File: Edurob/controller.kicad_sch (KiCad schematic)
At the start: 9 parts, among them SW1 SW_Push, U4 ESP32-S3-WROOM-1

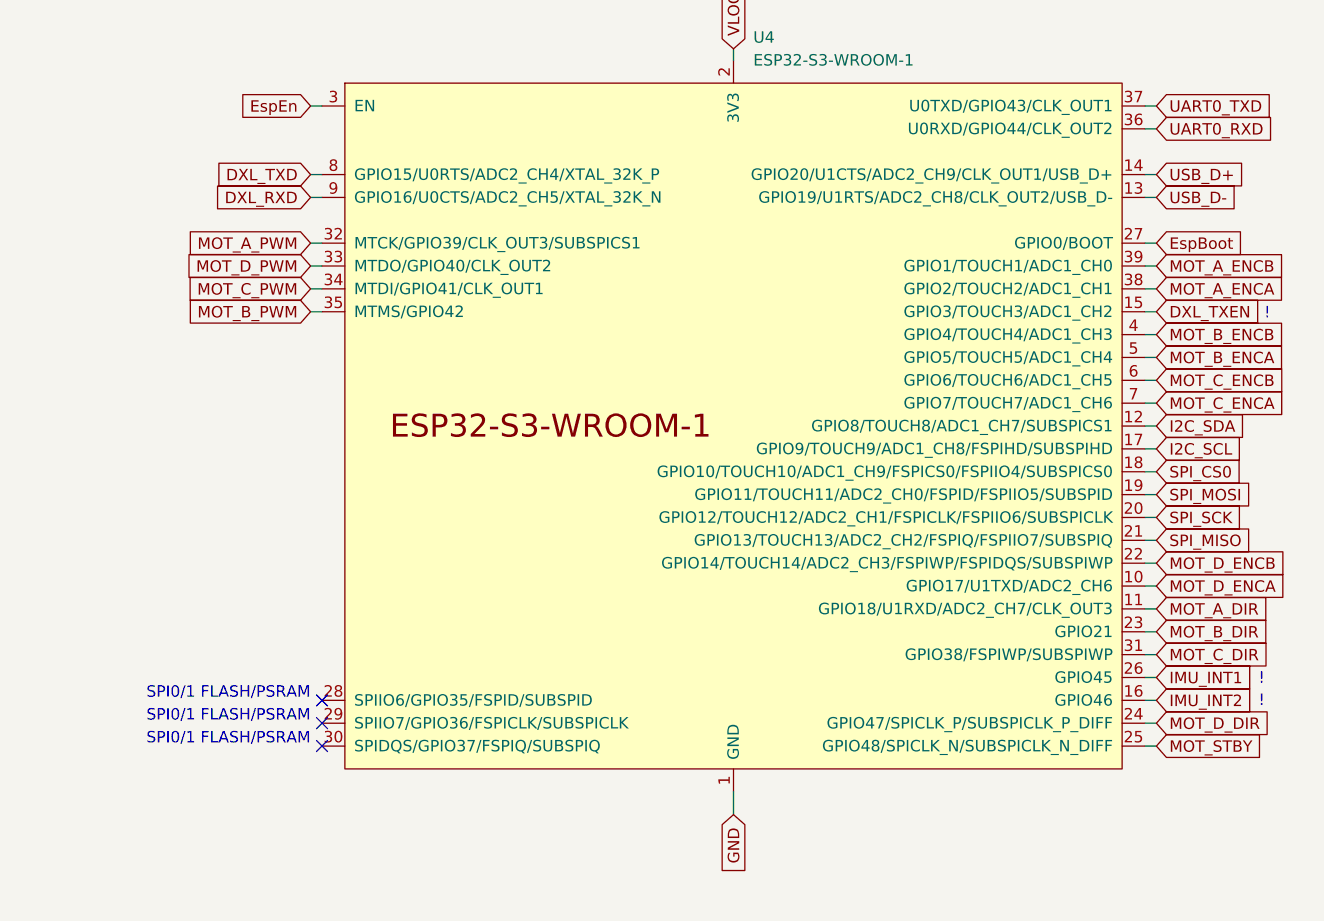
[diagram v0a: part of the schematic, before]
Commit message: Finalized part placement
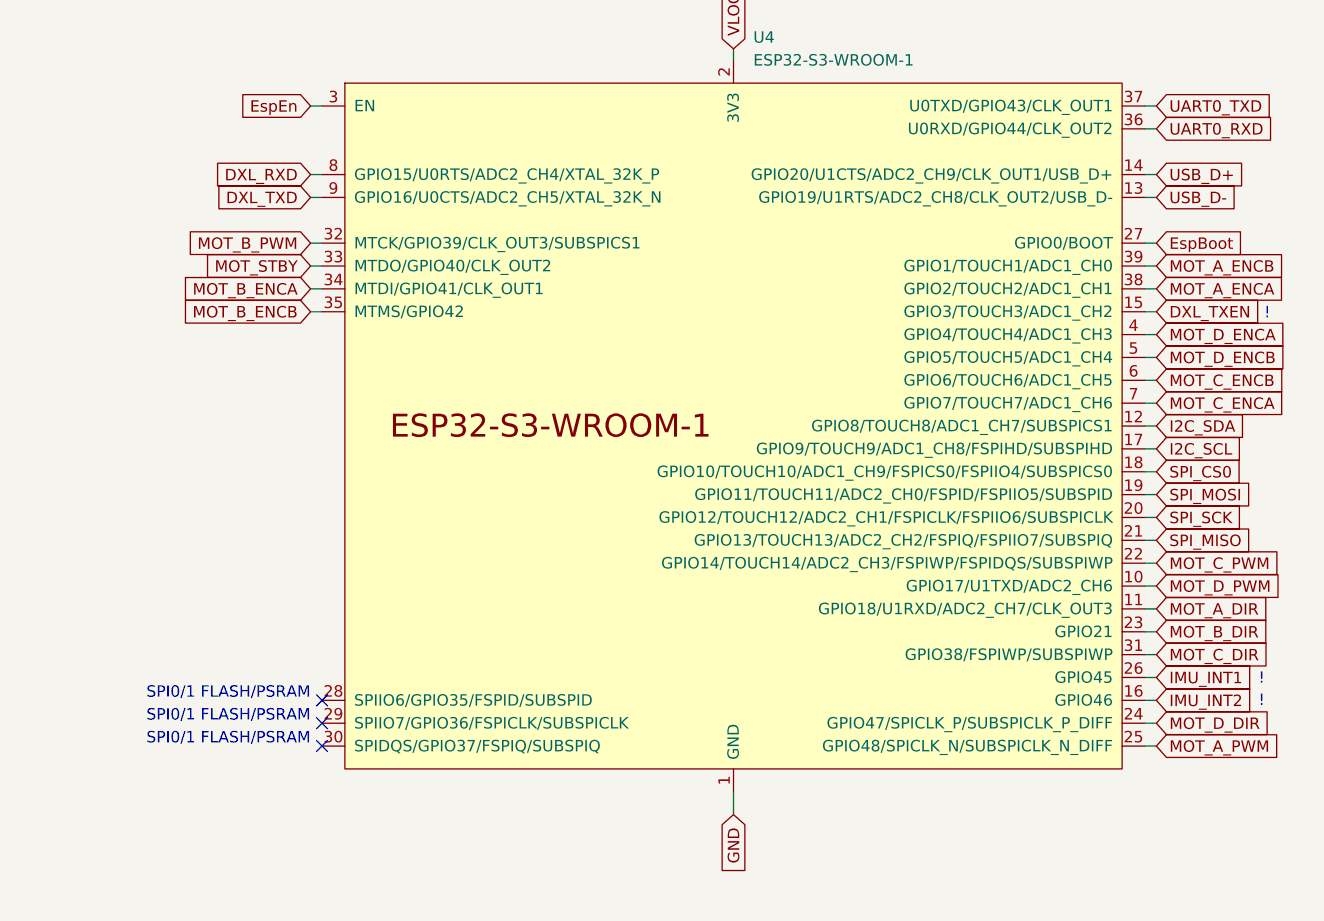
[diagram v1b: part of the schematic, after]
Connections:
- net DXL_RXD: now also U4.8 (GPIO15/U0RTS/ADC2_CH4/XTAL_32K_P); no longer U4.9 (GPIO16/U0CTS/ADC2_CH5/XTAL_32K_N)
- net DXL_TXD: now also U4.9 (GPIO16/U0CTS/ADC2_CH5/XTAL_32K_N); no longer U4.8 (GPIO15/U0RTS/ADC2_CH4/XTAL_32K_P)
- net MOT_A_PWM: now also U4.25 (GPIO48/SPICLK_N/SUBSPICLK_N_DIFF); no longer U4.32 (MTCK/GPIO39/CLK_OUT3/SUBSPICS1)
- net MOT_B_ENCA: now also U4.34 (MTDI/GPIO41/CLK_OUT1); no longer U4.5 (GPIO5/TOUCH5/ADC1_CH4)
- net MOT_B_ENCB: now also U4.35 (MTMS/GPIO42); no longer U4.4 (GPIO4/TOUCH4/ADC1_CH3)
- net MOT_B_PWM: now also U4.32 (MTCK/GPIO39/CLK_OUT3/SUBSPICS1); no longer U4.35 (MTMS/GPIO42)
- net MOT_C_PWM: now also U4.22 (GPIO14/TOUCH14/ADC2_CH3/FSPIWP/FSPIDQS/SUBSPIWP); no longer U4.34 (MTDI/GPIO41/CLK_OUT1)
- net MOT_D_ENCA: now also U4.4 (GPIO4/TOUCH4/ADC1_CH3); no longer U4.10 (GPIO17/U1TXD/ADC2_CH6)
- net MOT_D_ENCB: now also U4.5 (GPIO5/TOUCH5/ADC1_CH4); no longer U4.22 (GPIO14/TOUCH14/ADC2_CH3/FSPIWP/FSPIDQS/SUBSPIWP)
- net MOT_D_PWM: now also U4.10 (GPIO17/U1TXD/ADC2_CH6); no longer U4.33 (MTDO/GPIO40/CLK_OUT2)
- net MOT_STBY: now also U4.33 (MTDO/GPIO40/CLK_OUT2); no longer U4.25 (GPIO48/SPICLK_N/SUBSPICLK_N_DIFF)
